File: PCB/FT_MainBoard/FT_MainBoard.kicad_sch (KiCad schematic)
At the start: 40 parts, among them SW1 SW_Push

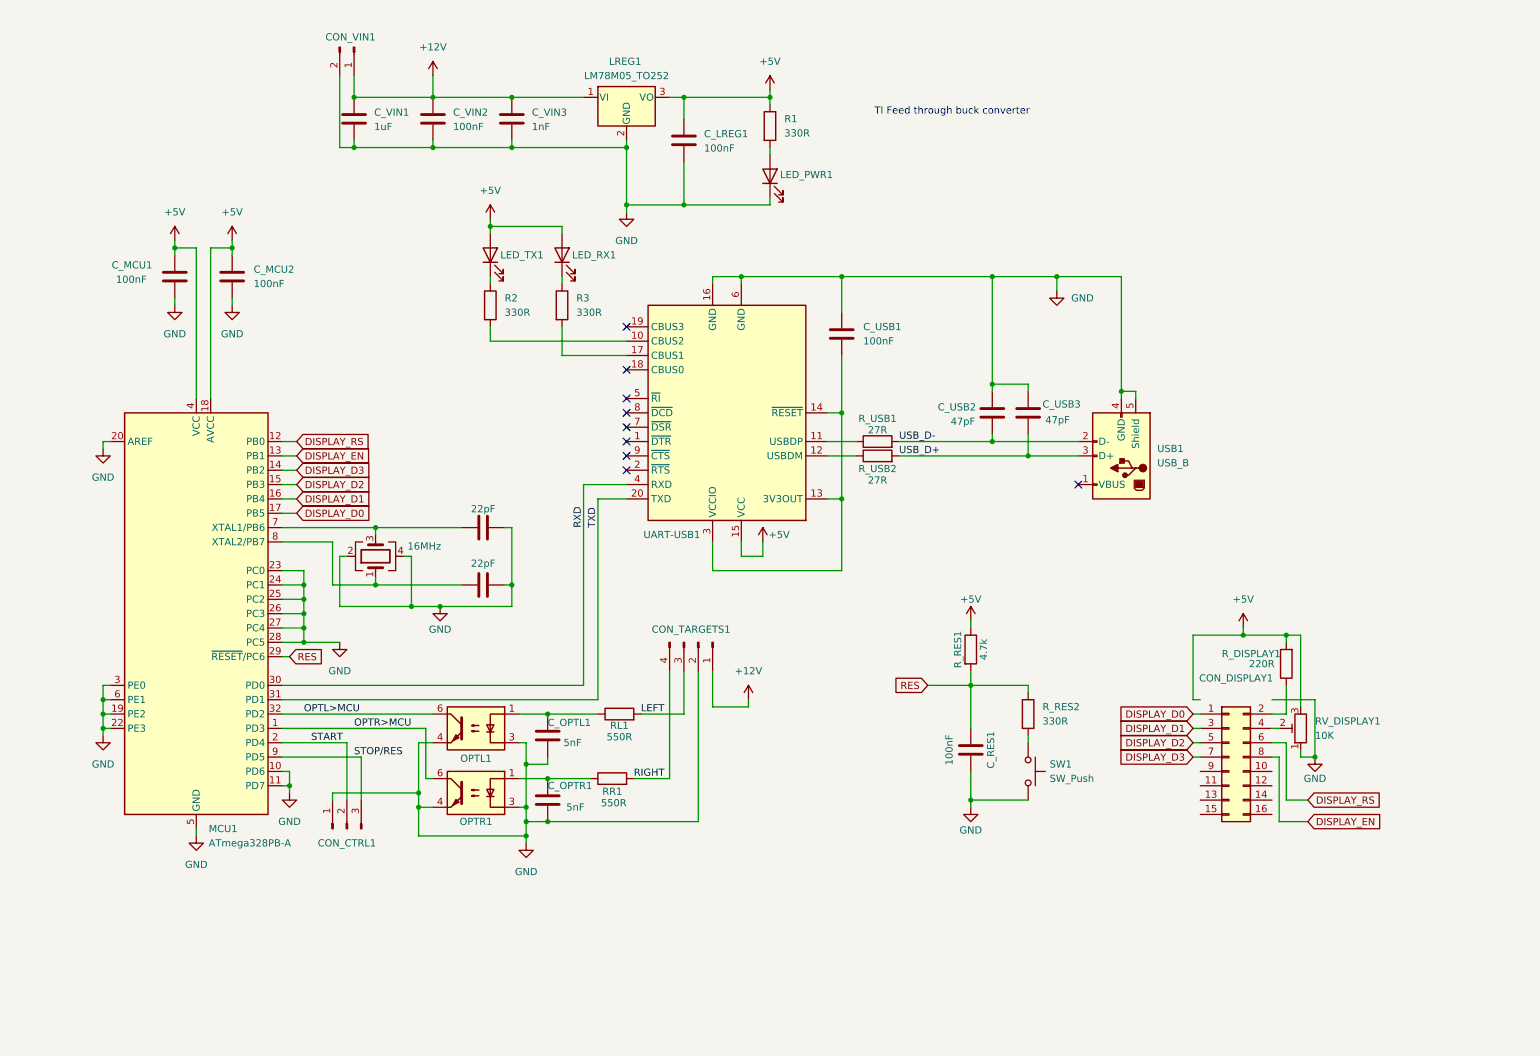
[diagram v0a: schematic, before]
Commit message: main board update
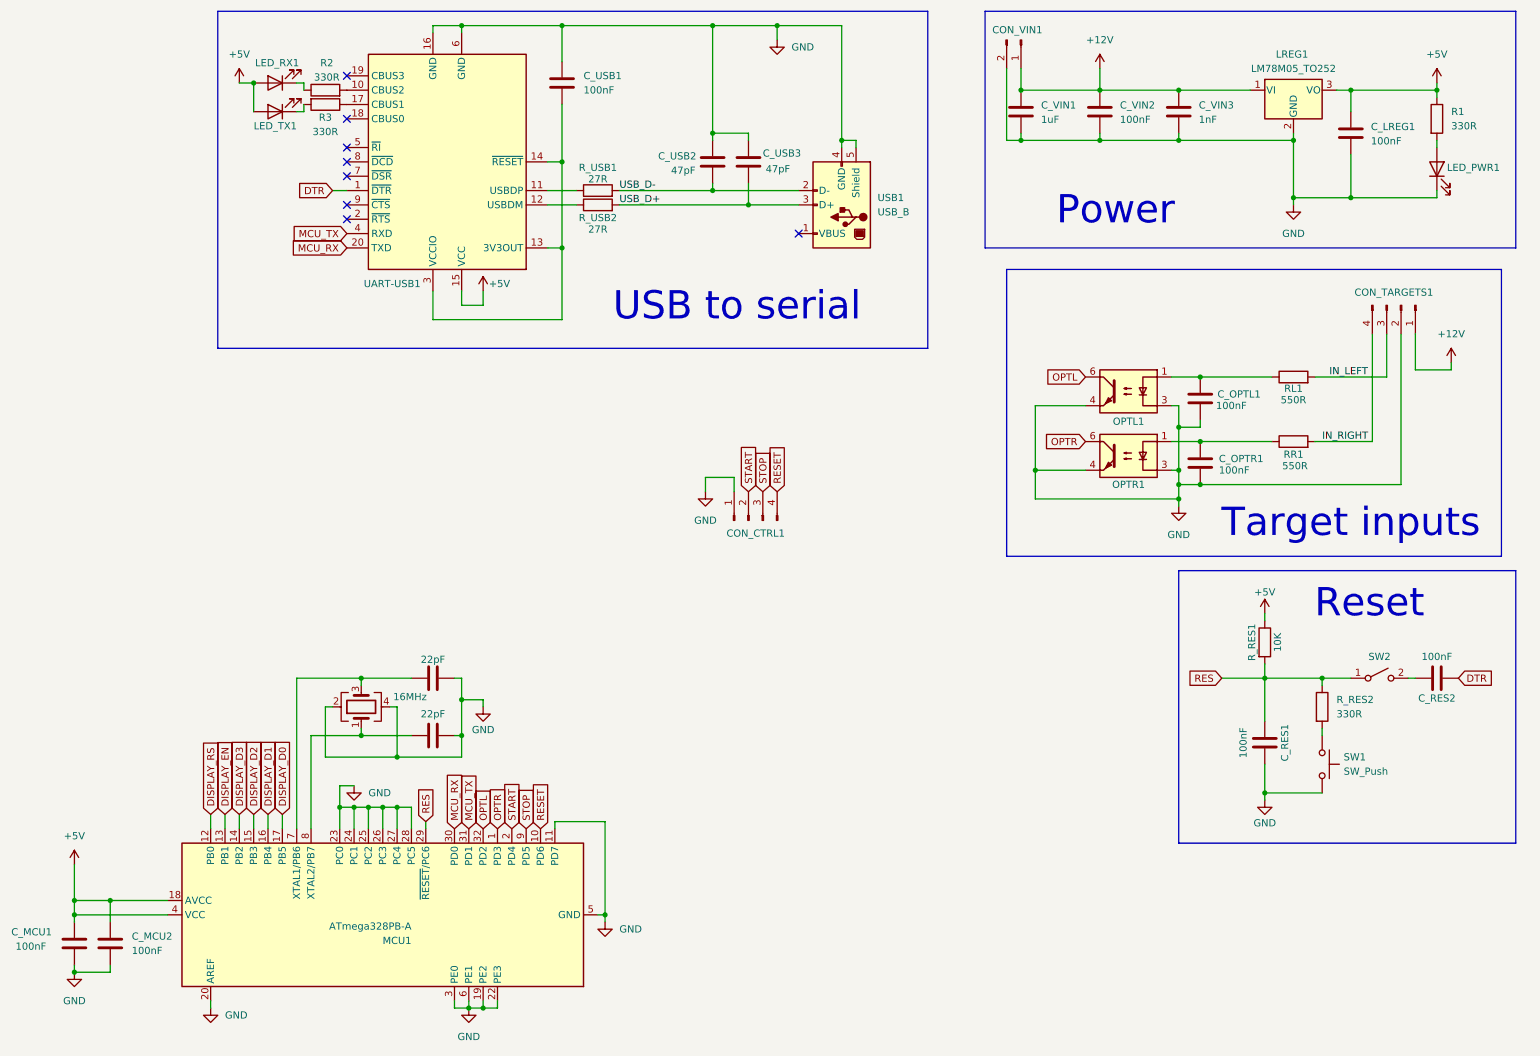
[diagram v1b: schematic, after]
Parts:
- removed CON_CTRL1: Conn_01x03_Pin, Connector_PinHeader_2.54mm:PinHeader_1x03_P2.54mm_Horizontal, symbol Connector:Conn_01x03_Pin
- removed CON_DISPLAY1: Conn_02x08_Odd_Even, Connector_PinHeader_2.54mm:PinHeader_2x08_P2.54mm_Vertical, symbol Connector_Generic:Conn_02x08_Odd_Even
- removed RV_DISPLAY1: 10K, Potentiometer_SMD:Potentiometer_Bourns_TC33X_Vertical, symbol Device:R_Potentiometer_Trim
- removed R_DISPLAY1: 220R, Resistor_SMD:R_0603_1608Metric, symbol Device:R
- added CON_CTRL1: Conn_01x04_Pin, Connector_PinHeader_2.54mm:PinHeader_1x04_P2.54mm_Horizontal, symbol Connector:Conn_01x04_Pin
- added C_RES2: 100nF, Capacitor_SMD:C_0603_1608Metric, symbol Device:C
- added SW2: SW_SPST, Button_Switch_THT:SW_DIP_SPSTx01_Slide_9.78x4.72mm_W7.62mm_P2.54mm, symbol Switch:SW_SPST
- C_OPTL1, C_OPTR1: value 5nF -> 100nF
- R_RES1: value 4.7k -> 10K
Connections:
- net GND: now also CON_CTRL1.1 (Pin_1); no longer MCU1.10 (PD6)
- net RES: now also SW2.1 (A)
- net START: now also CON_CTRL1.2 (Pin_2)
- net at LED_TX1.1 (K): now also R3.2; no longer R2.1
- net at LED_RX1.1 (K): now also R2.1; no longer R3.1
- net at UART-USB1.17 (CBUS1): now also R3.1; no longer R3.2
- net DTR: now reaches UART-USB1.1 (~{DTR})
- net DTR: now also C_RES2.1
- net LEFT renamed IN_LEFT
- net OPTL>MCU renamed OPTL
- net OPTR>MCU renamed OPTR
- net RIGHT renamed IN_RIGHT
- net RXD renamed MCU_RX
- net MCU_RX: now also UART-USB1.20 (TXD); no longer UART-USB1.4 (RXD)
- net STOP/RES renamed STOP
- net STOP: now also CON_CTRL1.3 (Pin_3)
- net TXD renamed MCU_TX
- net MCU_TX: now also UART-USB1.4 (RXD); no longer UART-USB1.20 (TXD)
- new net: C_RES2.2, SW2.2 (B)
- new net RESET: CON_CTRL1.4 (Pin_4), MCU1.10 (PD6)
- no-connect marks 9 -> 8
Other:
- note added: "Power"
- note added: "Reset"
- note added: "Target inputs"
- note added: "USB to serial"
- note removed: "TI Feed through buck converter"
- moved on the sheet: CON_TARGETS1, CON_VIN1, C_LREG1, C_MCU1, C_MCU2, C_OPTL1, C_OPTR1, C_RES1, C_USB1, C_USB2, C_USB3, C_VIN1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

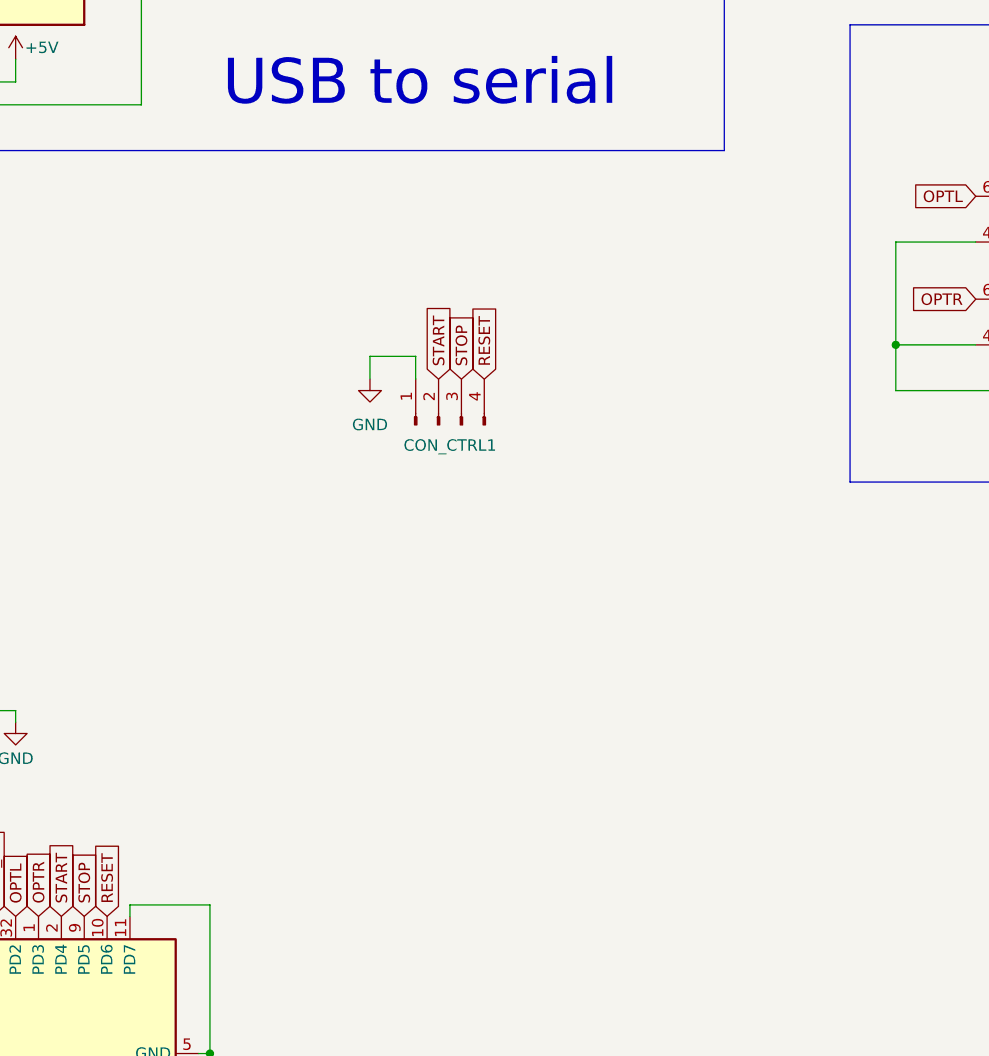
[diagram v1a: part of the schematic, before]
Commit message: main board update
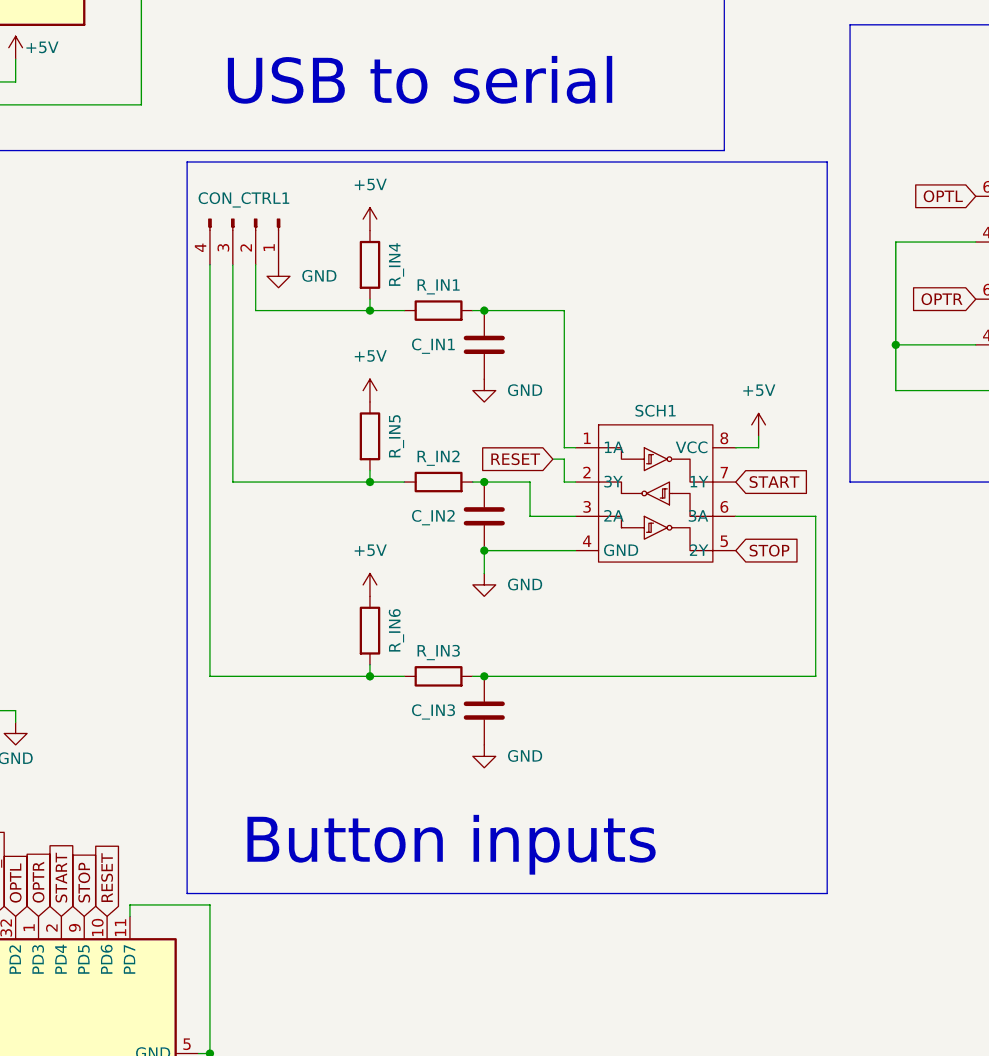
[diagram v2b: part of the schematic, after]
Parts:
- added C_IN1, C_IN2, C_IN3: 100n, Capacitor_SMD:C_0603_1608Metric, symbol Device:C
- added R_IN1, R_IN2, R_IN3, R_IN4, R_IN5, R_IN6: 1000R, Resistor_SMD:R_0603_1608Metric, symbol Device:R
- added SCH1: 74HC3G14DP,125, Package_SO:MSOP-8_3x3mm_P0.65mm, symbol 74HC3G14DP,125:74HC3G14DP,125
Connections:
- net +5V: now also R_IN4.1, R_IN5.1, R_IN6.1, SCH1.8 (VCC)
- net GND: now also C_IN1.2, C_IN2.2, C_IN3.2, SCH1.4 (GND)
- net RESET: now also SCH1.2 (3Y); no longer CON_CTRL1.4 (Pin_4)
- net START: now also SCH1.7 (1Y); no longer CON_CTRL1.2 (Pin_2)
- net STOP: now also SCH1.5 (2Y); no longer CON_CTRL1.3 (Pin_3)
- new net: CON_CTRL1.4 (Pin_4), R_IN3.1, R_IN6.2
- new net: C_IN3.1, R_IN3.2, SCH1.6 (3A)
- new net: CON_CTRL1.2 (Pin_2), R_IN1.1, R_IN4.2
- new net: CON_CTRL1.3 (Pin_3), R_IN2.1, R_IN5.2
- new net: C_IN1.1, R_IN1.2, SCH1.1 (1A)
- new net: C_IN2.1, R_IN2.2, SCH1.3 (2A)
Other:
- note added: "Button inputs"
- moved on the sheet: CON_CTRL1
